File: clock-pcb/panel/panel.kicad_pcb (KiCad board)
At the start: 2 copper layers, 90.3 x 97.4 mm, 144 parts, among them IC1 VEML6030-GS15, IC2 MCP23018-E_MJ, J1 Conn_01x03_Pin, J1 Conn_01x04_Socket, J1 Conn_01x07_Socket, J1 USB4145-03-0070-C, J11 Conn_01x06_Socket, J15 Conn_01x02_Socket, J2 Conn_01x04_Socket, J2 oled 2, J3 Led display, J4 Led display 2, J5 Conn_01x07_Socket, J6 Conn_01x07_Socket, J7 SFV25R-2STE1HLF, J8 Conn_01x04_Socket, J8 SFV25R-2STE1HLF, J9 Conn_01x04_Socket, U1 BMP280, U1 CC56-12EWA, U1 ESP32-C6-MINI-1-N4, U1 TMAG5231C1GQDBZR, U2 AS1115-BSST, U4 SHT4x, U4 TPS2116DRL, U5 MCP73811T-420I-OT, U6 TPS61040DBV, U7 TLV75533PDBV, U8 AT42QT2120-MMHR, Y2 32.768KHz

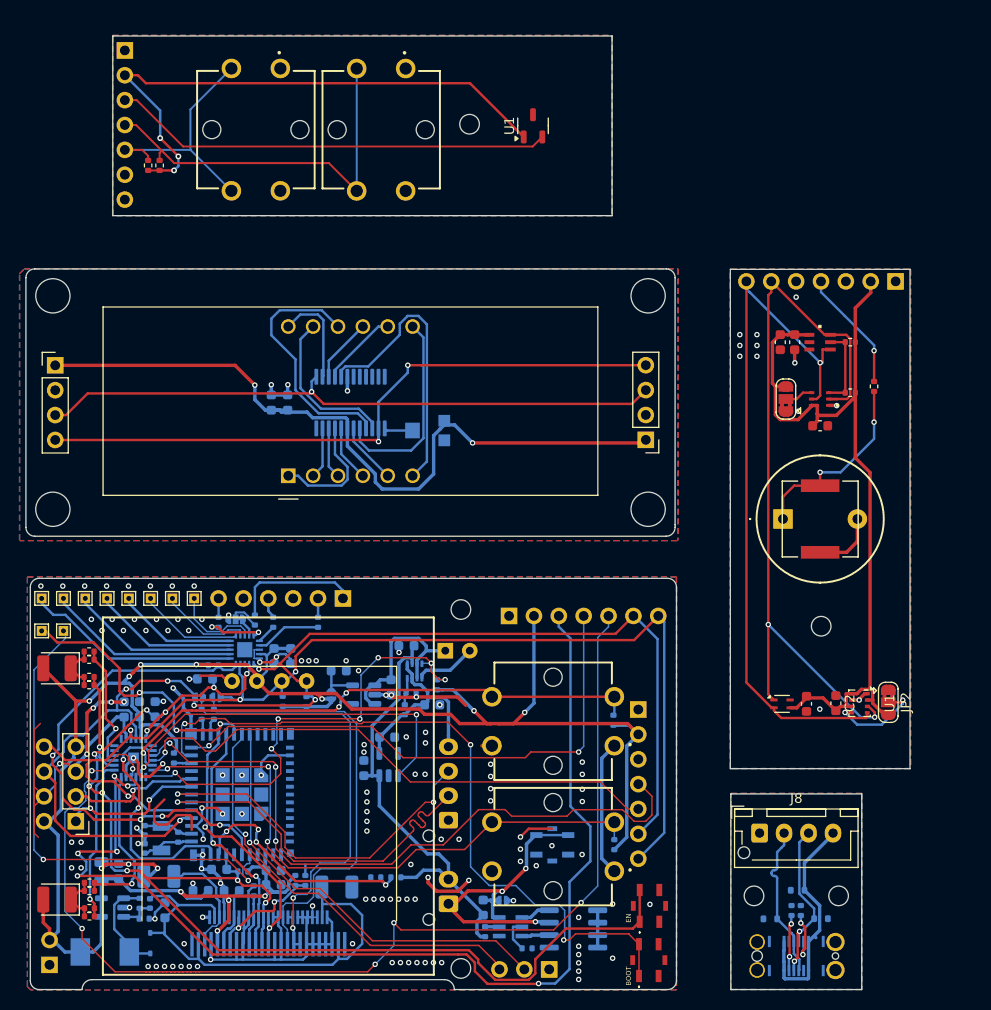
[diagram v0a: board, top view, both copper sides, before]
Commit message: panel
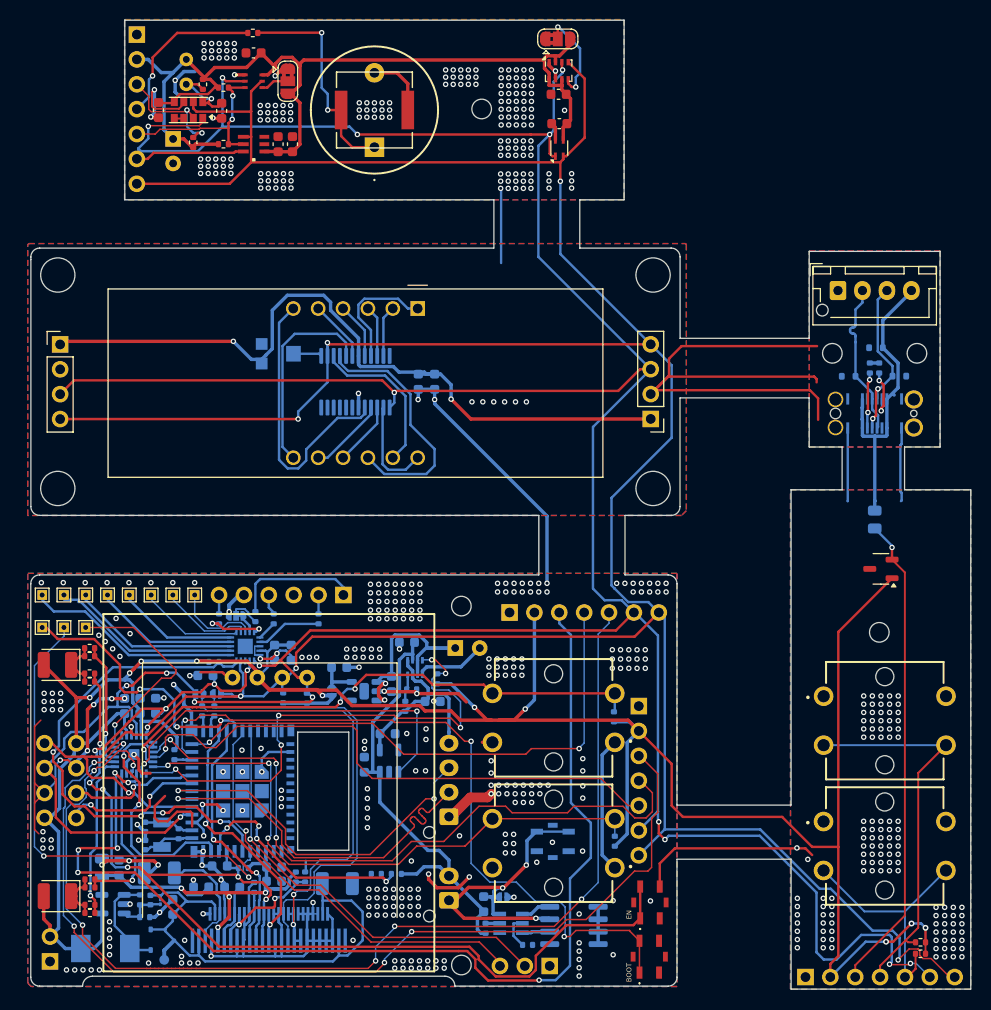
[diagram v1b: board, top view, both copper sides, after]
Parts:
- removed the C1 at (171.9, 90.5)
- removed the C1 at (116.2, 114.0)
- removed the C13 at (110.5, 135.8)
- removed the C2 at (173.5, 118.8)
- removed the C2 at (100.8, 119.5)
- removed the C23 at (117.5, 88.1)
- removed the C23 at (116.1, 135.9)
- removed the C24 at (115.9, 88.1)
- removed the C24 at (116.1, 137.4)
- removed the C3 at (169.3, 82.0)
- removed the C3 at (102.4, 119.5)
- removed the C4 at (167.9, 82.0)
- removed the C4 at (137.5, 139.7)
- removed the C5 at (133.6, 113.5)
- removed the C6 at (170.5, 118.9)
- removed the C6 at (132.3, 119.0)
- removed the C7 at (129.7, 113.0)
- removed the D1 at (94.0, 138.9)
- removed the D1 at (169.6, 138.0)
- removed the D2 at (94.0, 115.3)
- removed the D2 at (166.8, 140.9)
- removed the D3 at (172.0, 140.9)
- removed the D3 at (103.5, 143.4)
- removed the J1 at (93.8, 84.3)
- removed the J1 at (144.3, 146.0)
- removed the J1 at (179.6, 75.8)
- removed the J1 at (100.9, 52.2)
- removed the J1 at (169.5, 144.7)
- removed the J2 at (102.7, 141.1)
- removed the J2 at (154.1, 91.9)
- removed the J8 at (165.8, 132.1)
- removed the J8 at (115.6, 143.1)
- removed the JP1 at (168.4, 87.8)
- removed the JP1 at (139.5, 139.0)
- removed the JP2 at (178.9, 118.8)
- removed the JP2 at (112.2, 110.3)
- removed the L1 at (168.1, 100.0)
- removed the L1 at (98.9, 144.0)
- removed the R1 at (104.5, 63.9)
- removed the R1 at (175.0, 87.1)
- removed the R1 at (117.0, 118.7)
- removed the R1 at (170.0, 140.0)
- removed the R11 at (103.3, 63.9)
- removed the R11 at (113.0, 136.0)
- removed the R2 at (175.0, 82.0)
- removed the R2 at (128.6, 136.6)
- removed the R3 at (126.5, 136.6)
- removed the R3 at (169.0, 140.0)
- removed the R4 at (177.4, 86.5)
- removed the R4 at (137.7, 142.2)
- removed the R5 at (142.0, 143.9)
- removed the R6 at (132.8, 117.0)
- removed the S1 at (114.3, 60.3)
- removed the S1 at (154.4, 145.1)
- removed the S2 at (154.5, 139.5)
- removed the S2 at (127.1, 60.3)
- removed the U1 at (117.6, 95.6)
- removed the U1 at (175.9, 118.8)
- removed the U1 at (142.6, 59.9)
- removed the U1 at (112.9, 128.2)
- removed the U2 at (171.9, 82.0)
- removed the U2 at (124.0, 88.1)
- removed the U2 at (140.3, 141.7)
- removed the U3 at (134.0, 139.3)
- removed the U4 at (168.0, 118.9)
- removed the U4 at (130.5, 115.5)
- added C1: 0.1uF, Capacitor_SMD:C_0603_1608Metric, F.Cu at (114.1, 52.4)
- added C1: 0.1uF, Capacitor_SMD:C_0603_1608Metric, B.Cu at (116.2, 113.7)
- added C13: 1uF, Capacitor_SMD:C_0603_1608Metric, F.Cu at (104.4, 58.3)
- added C13: 1uF, Capacitor_SMD:C_0603_1608Metric, B.Cu at (110.6, 135.5)
- added C2: 0.1uF, Capacitor_SMD:C_0603_1608Metric, F.Cu at (145.2, 56.6)
- added C2: 0.1uF, Capacitor_SMD:C_0603_1608Metric, B.Cu at (100.9, 119.1)
- added C22: 6.4pF, Capacitor_SMD:C_01005_0402Metric, B.Cu at (104.5, 139.1)
- added C23: 0.1uF, Capacitor_SMD:C_0603_1608Metric, B.Cu at (130.9, 86.0)
- added C23: 0.1uF, Capacitor_SMD:C_0603_1608Metric, B.Cu at (116.2, 135.6)
- added C24: 10uF, Capacitor_SMD:C_0603_1608Metric, B.Cu at (116.2, 137.0)
- added C24: 10uF, Capacitor_SMD:C_0603_1608Metric, B.Cu at (132.6, 86.0)
- added C3: 0.1uF, Capacitor_SMD:C_0603_1608Metric, F.Cu at (116.6, 61.7)
- added C3: 10uF, Capacitor_SMD:C_0603_1608Metric, B.Cu at (102.5, 119.1)
- added C4: 4.7uF, Capacitor_SMD:C_0603_1608Metric, F.Cu at (118.0, 61.7)
- added C4: 0.1uF, Capacitor_SMD:C_0603_1608Metric, B.Cu at (137.6, 139.4)
- added C5: 1uF, Capacitor_SMD:C_0603_1608Metric, F.Cu at (110.8, 58.3)
- added C5: 100uF, Capacitor_THT:CP_Radial_D5.0mm_P2.50mm, B.Cu at (134.7, 113.2)
- added C6: 0.1uF, Capacitor_SMD:C_0603_1608Metric, F.Cu at (145.3, 59.6)
- added C6: 1uF, Capacitor_SMD:C_0603_1608Metric, B.Cu at (132.4, 118.7)
- added C7: 1uF, Capacitor_SMD:C_0603_1608Metric, B.Cu at (129.7, 112.6)
- added C7: 100uF, Capacitor_THT:CP_Radial_D5.0mm_P2.50mm, B.Cu at (105.8, 61.2)
- added D1: LED, LED_SMD:LED_1210_3225Metric, F.Cu at (94.0, 138.6)
- added D1: ESD5Zxx, Diode_SMD:D_SOD-523, B.Cu at (177.6, 82.5)
- added D2: LED, LED_SMD:LED_1210_3225Metric, F.Cu at (94.0, 114.9)
- added D2: ESD5Zxx, Diode_SMD:D_SOD-523, B.Cu at (174.8, 85.5)
- added D3: NSVR0340HT1G, Diode_SMD:D_SOD-323, B.Cu at (103.6, 143.0)
- added D3: ESD5Zxx, Diode_SMD:D_SOD-523, B.Cu at (180.0, 85.4)
- added J1: Conn_01x04_Socket, Connector_PinHeader_2.54mm:PinHeader_1x04_P2.54mm_Vertical, F.Cu at (154.6, 89.8)
- added J1: Conn_01x07_Socket, Connector_PinHeader_2.54mm:PinHeader_1x07_P2.54mm_Horizontal, B.Cu at (102.1, 50.5)
- added J1: Conn_01x07_Socket, Connector_PinHeader_2.54mm:PinHeader_1x07_P2.54mm_Horizontal, B.Cu at (170.4, 146.8)
- added J1: Conn_01x03_Pin, Connector_PinHeader_2.54mm:PinHeader_1x03_P2.54mm_Vertical, B.Cu at (144.3, 145.7)
- added J1: USB4145-03-0070-C, clock:USB4145030070C, B.Cu at (177.5, 89.2)
- added J2: Conn_01x04_Socket, Connector_PinHeader_2.54mm:PinHeader_1x04_P2.54mm_Vertical, F.Cu at (94.3, 82.2)
- added J2: oled 2, clock:SSD1306_0.96_Oled, F.Cu at (102.7, 140.7)
- added J8: Conn_01x04_Socket, Connector_JST:JST_XH_B4B-XH-AM_1x04_P2.50mm_Vertical, F.Cu at (173.8, 76.7)
- added J8: SFV25R-2STE1HLF, clock:AMPHENOL_SFV25R-2STE1HLF, B.Cu at (115.6, 142.8)
- added JP1: SolderJumper_3_Bridged12, Jumper:SolderJumper-3_P1.3mm_Bridged2Bar12_RoundedPad1.0x1.5mm, F.Cu at (117.6, 55.3)
- added JP1: Jumper, clock:jumper_solder_small, B.Cu at (139.6, 138.7)
- added JP2: SolderJumper_3_Bridged12, Jumper:SolderJumper-3_P1.3mm_Bridged2Bar12_RoundedPad1.0x1.5mm, F.Cu at (145.1, 51.0)
- added JP2: SolderJumper_3_Bridged12, clock:jumper_solder_small_3_bridged, B.Cu at (112.3, 109.9)
- added L1: CPT-14146-80T, clock:CPT1414680T, F.Cu at (126.4, 62.1)
- added L1: 10uH 1A, clock:HPI0530-100, B.Cu at (98.9, 143.7)
- added R1: 10K, Resistor_SMD:R_0402_1005Metric, F.Cu at (182.2, 143.3)
- added R1: 10K, Resistor_SMD:R_0402_1005Metric, F.Cu at (111.0, 56.0)
- added R1: 100k, Resistor_SMD:R_0402_1005Metric, B.Cu at (117.1, 118.3)
- added R1: 5.1k, Resistor_SMD:R_0402_1005Metric, B.Cu at (178.0, 84.6)
- added R11: 10K, Resistor_SMD:R_0402_1005Metric, F.Cu at (182.2, 144.4)
- added R11: 10K, Resistor_SMD:R_0402_1005Metric, B.Cu at (113.0, 135.7)
- added R2: 10K, Resistor_SMD:R_0402_1005Metric, F.Cu at (111.0, 61.7)
- added R2: 300k, Resistor_SMD:R_0402_1005Metric, B.Cu at (128.6, 136.3)
- added R3: 10K, Resistor_SMD:R_0402_1005Metric, F.Cu at (107.9, 61.6)
- added R3: 5.1k, Resistor_SMD:R_0402_1005Metric, B.Cu at (177.0, 84.6)
- added R3: 800k, Resistor_SMD:R_0402_1005Metric, B.Cu at (126.6, 136.3)
- added R4: 330R, Resistor_SMD:R_0402_1005Metric, F.Cu at (114.0, 50.4)
- added R4: 330R, Resistor_SMD:R_0402_1005Metric, B.Cu at (137.8, 141.8)
- added R5: 22R, Resistor_SMD:R_0402_1005Metric, F.Cu at (108.9, 55.6)
- added R5: 2.7K, Resistor_SMD:R_0402_1005Metric, B.Cu at (142.0, 143.5)
- added R6: 10K, Resistor_SMD:R_0402_1005Metric, B.Cu at (132.8, 116.4)
- added R6: 22R, Resistor_THT:R_Axial_DIN0204_L3.6mm_D1.6mm_P2.54mm_Vertical, B.Cu at (107.2, 53.1)
- added REF**: R_0805_2012Metric, Resistor_SMD:R_0805_2012Metric, B.Cu at (177.5, 100.1)
- added S1: B3F-5050, clock:B3F-4055, F.Cu at (178.5, 133.4)
- added S1: TS21-34-035-BK-160-SMT-TR, clock:TS2134035BK160SMTTR, F.Cu at (154.5, 144.7)
- added S2: B3F-5050, clock:B3F-4055, F.Cu at (178.5, 120.6)
- added S2: TS21-34-035-BK-160-SMT-TR, clock:TS2134035BK160SMTTR, F.Cu at (154.5, 139.2)
- added TP10: TestPoint, TestPoint:TestPoint_THTPad_1.0x1.0mm_Drill0.5mm, F.Cu at (96.9, 111.1)
- added TP2: TestPoint, TestPoint:TestPoint_Pad_D1.0mm, B.Cu at (104.9, 145.1)
- added U1: BMP280, clock:Bosch_LGA-8_2x2.5mm_P0.65mm_ClockwisePinNumbering, F.Cu at (145.2, 54.2)
- added U1: CC56-12EWA, Display_7Segment:CA56-12EWA, F.Cu at (130.8, 78.5)
- added U1: TMAG5231C1GQDBZR, Package_TO_SOT_SMD:SOT-23-3, F.Cu at (178.1, 105.1)
- added U1: ESP32-C6-MINI-1-N4, clock:XCVR_ESP32-C6-MINI-1-N4, B.Cu at (112.9, 127.8)
- added U2: ~, clock:LTR-F216A, F.Cu at (114.1, 61.7)
- added U2: AS1115-BSST, Package_SO:QSOP-24_3.9x8.7mm_P0.635mm, B.Cu at (124.5, 86.0)
- added U2: ~, clock:SOT95P280X140-6N, B.Cu at (140.4, 141.3)
- added U3: APDS-9960, clock:Avago_APDS-9960, F.Cu at (107.4, 58.3)
- added U3: ~, Connector_JST:JST_XH_B2B-XH-AM_1x02_P2.50mm_Vertical, B.Cu at (134.0, 139.0)
- added U4: SHT4x, clock:Sensirion_DFN-4_1.5x1.5mm_P0.8mm_SHT4x_NoCentralPad, F.Cu at (145.3, 62.1)
- added U4: TPS2116DRL, Package_TO_SOT_SMD:SOT-583-8, B.Cu at (130.6, 115.2)
- J4: footprint Connector_PinHeader_2.54mm:PinHeader_1x04_P2.54mm_Vertical -> clock:PinHeader_1x04_P2.54mm_Vertical
- U7: footprint Package_TO_SOT_SMD:SOT-23-5 -> clock:TLV75733PDYDR
- moved IC1 66.4 mm to (114.1, 55.3), turned to 0 degrees
- moved LS1 61.8 mm to (126.4, 58.3), turned to 0 degrees
- moved VR1 17.0 mm to (116.7, 83.2), turned to 90 degrees
- moved C17 0.88 mm to (105.8, 139.6)
- moved R30 0.36 mm to (119.3, 136.6)
- moved C16 0.35 mm to (98.6, 135.7)
- moved C19 0.35 mm to (103.0, 131.5)
- moved C20 0.35 mm to (103.0, 133.3)
- moved C27 0.35 mm to (122.6, 137.3)
- moved R18 0.35 mm to (97.3, 140.3)
- moved S4 0.35 mm to (144.7, 133.1)
- moved S5 0.35 mm to (144.6, 133.0)
- moved C18 0.35 mm to (103.5, 139.0)
- moved AO9926C1 0.35 mm to (146.8, 141.5)
- moved C11 0.35 mm to (125.4, 125.1)
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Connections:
- IC1 pad 3: GPIO25 -> SUB_TOP_1
- IC2 pad 13: unconnected-(IC2-INTB-Pad13) -> INT_A
- IC2 pad 4: unconnected-(IC2-GPB4-Pad4) -> HALL_SENS
- IC2 pad 6: unconnected-(IC2-GPB6-Pad6) -> Net-(IC2-GPB6)
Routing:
- net GND: track 205.9 -> 352.4 mm, vias 146 -> 593
- net SDA: track 275.6 -> 382.7 mm, vias 9 -> 16
- net HALL_SENS: track 45.0 -> 151.8 mm, vias 0 -> 6
- net SCL: track 260.0 -> 354.0 mm, vias 7 -> 8
- net +3V3: track 364.7 -> 407.2 mm
- net Net-(IC2-GPB6): track 0.00 -> 21.5 mm, vias 0 -> 1
- net SUB_TOP_1: track 114.5 -> 131.8 mm, vias 6 -> 8
- net SUB_TOP_3: track 112.7 -> 124.5 mm, vias 6 -> 8
- net GPIO25: track 8.37 -> 0.00 mm
- net Net-(U3-VDD): track 0.00 -> 7.86 mm, vias 0 -> 1
- net VBUS: track 43.5 -> 51.1 mm
- net POWER_STATUS: track 46.7 -> 51.7 mm, vias 7 -> 6
- net BUZZER: track 68.6 -> 72.8 mm
- net 14V_OLED: track 48.5 -> 51.7 mm
- net BUZZER_IN: track 19.7 -> 22.6 mm
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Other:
- board size 90.3 x 97.4 mm -> 96 x 99 mm
